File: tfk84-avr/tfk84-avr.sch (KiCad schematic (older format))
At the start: 31 parts, among them J1 USB_C_Receptacle_USB2.0, J2 AVR-ISP-6, SW1 Reset, U1 ATmega32U4-AU, Y1 16MHz

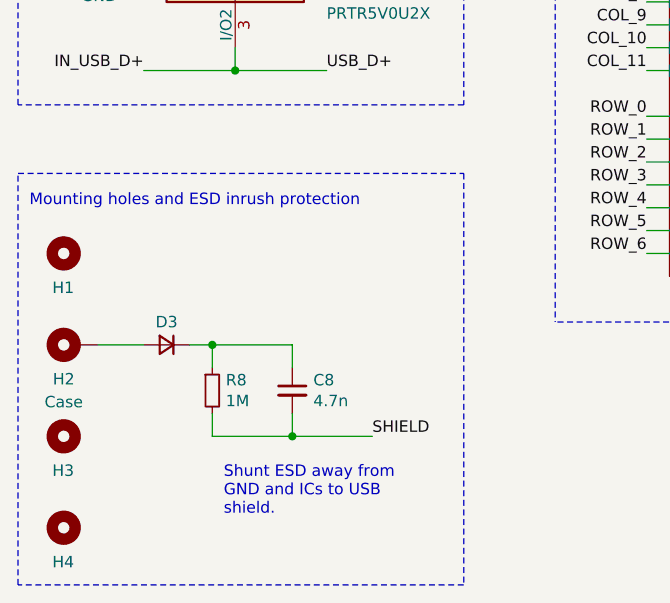
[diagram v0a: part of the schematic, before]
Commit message: Continue layout
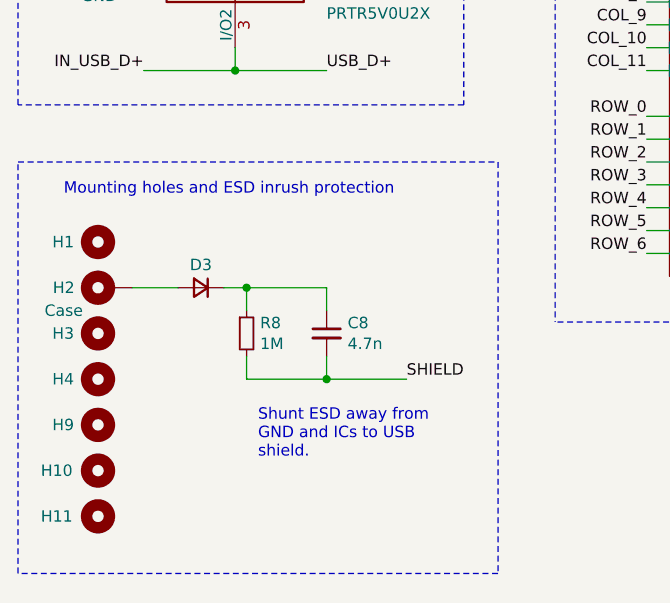
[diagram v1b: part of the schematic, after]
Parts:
- added H10, H11, H9: MountingHole, MountingHole:MountingHole_2.5mm_Pad, symbol Mechanical:MountingHole
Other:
- moved on the sheet: C8, D3, H1, H2, H3, H4, R8
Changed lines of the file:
@@
 L Device:D_Small D3
 U 1 1 60989164
-P 1350 6550
+P 1500 6300
 AR Path="/60989164" Ref="D3"  Part="1"
 AR Path="/60815FFC/60989164" Ref="D?"  Part="1"
-F 0 "D3" H 1350 6450 50  0000 C CNN
-F 1 "Case ESD" H 1350 6434 50  0001 C CNN
-F 2 "Diode_SMD:D_SOD-123" V 1350 6550 50  0001 C CNN
-F 3 "~" V 1350 6550 50  0001 C CNN
-	1    1350 6550
+F 0 "D3" H 1500 6200 50  0000 C CNN
+F 1 "Case ESD" H 1500 6184 50  0001 C CNN
+F 2 "Diode_SMD:D_SOD-123" V 1500 6300 50  0001 C CNN
+F 3 "~" V 1500 6300 50  0001 C CNN
+	1    1500 6300
 	-1   0    0    1
 $EndComp
 Wire Wire Line
-	1450 6550 1550 6550
-Wire Wire Line
-	1550 6550 1550 6650
-Wire Wire Line
-	1550 6550 1900 6550
-Wire Wire Line
-	1900 6550 1900 6650
-Connection ~ 1550 6550
+	1600 6300 1700 6300
+Wire Wire Line
+	1700 6300 1700 6400
+Wire Wire Line
+	1700 6300 2050 6300
+Wire Wire Line
+	2050 6300 2050 6400
+Connection ~ 1700 6300
 $Comp
 L Device:R_Small R8
 U 1 1 6098916F
-P 1550 6750
+P 1700 6500
 AR Path="/6098916F" Ref="R8"  Part="1"
 AR Path="/60815FFC/6098916F" Ref="R?"  Part="1"
-F 0 "R8" H 1609 6796 50  0000 L CNN
-F 1 "1M" H 1609 6705 50  0000 L CNN
-F 2 "Resistor_SMD:R_0805_2012Metric_Pad1.20x1.40mm_HandSolder" H 1550 6750 50  0001 C CNN
-F 3 "~" H 1550 6750 50  0001 C CNN
-	1    1550 6750
+F 0 "R8" H 1759 6546 50  0000 L CNN
+F 1 "1M" H 1759 6455 50  0000 L CNN
+F 2 "Resistor_SMD:R_0805_2012Metric_Pad1.20x1.40mm_HandSolder" H 1700 6500 50  0001 C CNN
+F 3 "~" H 1700 6500 50  0001 C CNN
+	1    1700 6500
 	1    0    0    -1
 $EndComp
@@
 L Device:C_Small C8
 U 1 1 60989175
-P 1900 6750
+P 2050 6500
 AR Path="/60989175" Ref="C8"  Part="1"
 AR Path="/60815FFC/60989175" Ref="C?"  Part="1"
-F 0 "C8" H 1992 6796 50  0000 L CNN
-F 1 "4.7n" H 1992 6705 50  0000 L CNN
-F 2 "Capacitor_SMD:C_0805_2012Metric_Pad1.18x1.45mm_HandSolder" H 1900 6750 50  0001 C CNN
-F 3 "~" H 1900 6750 50  0001 C CNN
-	1    1900 6750
-	1    0    0    -1
-$EndComp
-Wire Wire Line
-	1900 6850 1900 6950
-Wire Wire Line
-	1900 6950 1550 6950
-Wire Wire Line
-	1550 6950 1550 6850
-Text Notes 750  5950 0    50   ~ 0
+F 0 "C8" H 2142 6546 50  0000 L CNN
+F 1 "4.7n" H 2142 6455 50  0000 L CNN
+F 2 "Capacitor_SMD:C_0805_2012Metric_Pad1.18x1.45mm_HandSolder" H 2050 6500 50  0001 C CNN
+F 3 "~" H 2050 6500 50  0001 C CNN
+	1    2050 6500
+	1    0    0    -1
+$EndComp
+Wire Wire Line
+	2050 6600 2050 6700
+Wire Wire Line
+	2050 6700 1700 6700
+Wire Wire Line
+	1700 6700 1700 6600
+Text Notes 900  5900 0    50   ~ 0
 Mounting holes and ESD inrush protection
 Wire Notes Line
-	700  5800 2650 5800
-Wire Notes Line
-	2650 5800 2650 7600
-Wire Notes Line
-	2650 7600 700  7600
-Wire Notes Line
-	700  7600 700  5800
-Wire Wire Line
-	1250 6550 1050 6550
+	700  5750 2800 5750
+Wire Notes Line
+	2800 5750 2800 7550
+Wire Notes Line
+	2800 7550 700  7550
+Wire Notes Line
+	700  7550 700  5750
+Wire Wire Line
+	1400 6300 1200 6300
 $Comp
 L Mechanical:MountingHole_Pad H2
 U 1 1 60989184
-P 950 6550
+P 1100 6300
 AR Path="/60989184" Ref="H2"  Part="1"
 AR Path="/60815FFC/60989184" Ref="H?"  Part="1"
-F 0 "H2" V 800 6600 50  0000 C CNN
-F 1 "Case" V 700 6600 50  0000 C CNN
-F 2 "MountingHole:MountingHole_2.5mm_Pad" H 950 6550 50  0001 C CNN
-F 3 "~" H 950 6550 50  0001 C CNN
-	1    950  6550
+F 0 "H2" V 1100 6500 50  0000 C CNN
+F 1 "Case" V 1000 6500 50  0000 C CNN
+F 2 "MountingHole:MountingHole_2.5mm_Pad" H 1100 6300 50  0001 C CNN
+F 3 "~" H 1100 6300 50  0001 C CNN
+	1    1100 6300
 	0    -1   -1   0
 $EndComp
 Wire Wire Line
-	1900 6950 2250 6950
-Connection ~ 1900 6950
-Text Label 2250 6950 0    50   ~ 0
+	2050 6700 2400 6700
+Connection ~ 2050 6700
+Text Label 2400 6700 0    50   ~ 0
 SHIELD
-Text Notes 1600 7300 0    50   ~ 0
+Text Notes 1750 7050 0    50   ~ 0
 Shunt ESD away from \nGND and ICs to USB \nshield.
 Wire Wire Line
@@
 L Mechanical:MountingHole H1
 U 1 1 60BC9C45
-P 900 6150
-F 0 "H1" H 850 6000 50  0000 L CNN
-F 1 "MountingHole" H 800 5900 50  0001 L CNN
-F 2 "MountingHole:MountingHole_2.5mm_Pad" H 900 6150 50  0001 C CNN
-F 3 "~" H 900 6150 50  0001 C CNN
-	1    900  6150
+P 1050 6100
+F 0 "H1" H 850 6100 50  0000 L CNN
+F 1 "MountingHole" H 950 5850 50  0001 L CNN
+F 2 "MountingHole:MountingHole_2.5mm_Pad" H 1050 6100 50  0001 C CNN
+F 3 "~" H 1050 6100 50  0001 C CNN
+	1    1050 6100
 	1    0    0    -1
 $EndComp
@@
 L Mechanical:MountingHole H3
 U 1 1 60BCA1EE
-P 900 6950
-F 0 "H3" H 850 6800 50  0000 L CNN
-F 1 "MountingHole" H 1000 6905 50  0001 L CNN
-F 2 "MountingHole:MountingHole_2.5mm_Pad" H 900 6950 50  0001 C CNN
-F 3 "~" H 900 6950 50  0001 C CNN
-	1    900  6950
+P 1050 6500
+F 0 "H3" H 850 6500 50  0000 L CNN
+F 1 "MountingHole" H 1150 6455 50  0001 L CNN
+F 2 "MountingHole:MountingHole_2.5mm_Pad" H 1050 6500 50  0001 C CNN
+F 3 "~" H 1050 6500 50  0001 C CNN
+	1    1050 6500
 	1    0    0    -1
 $EndComp
@@
 L Mechanical:MountingHole H4
 U 1 1 60BCA526
-P 900 7350
-F 0 "H4" H 850 7200 50  0000 L CNN
-F 1 "MountingHole" H 1000 7305 50  0001 L CNN
-F 2 "MountingHole:MountingHole_2.5mm_Pad" H 900 7350 50  0001 C CNN
-F 3 "~" H 900 7350 50  0001 C CNN
-	1    900  7350
+P 1050 6700
+F 0 "H4" H 850 6700 50  0000 L CNN
+F 1 "MountingHole" H 1150 6655 50  0001 L CNN
+F 2 "MountingHole:MountingHole_2.5mm_Pad" H 1050 6700 50  0001 C CNN
+F 3 "~" H 1050 6700 50  0001 C CNN
+	1    1050 6700
 	1    0    0    -1
 $EndComp
@@
 Text Label 10150 4650 0    50   ~ 0
 COL_11
+$Comp
+L Mechanical:MountingHole H9
+U 1 1 60FF3666
+P 1050 6900
+F 0 "H9" H 850 6900 50  0000 L CNN
+F 1 "MountingHole" H 1150 6855 50  0001 L CNN
+F 2 "MountingHole:MountingHole_2.5mm_Pad" H 1050 6900 50  0001 C CNN
+F 3 "~" H 1050 6900 50  0001 C CNN
+	1    1050 6900
+	1    0    0    -1
+$EndComp
+$Comp
+L Mechanical:MountingHole H10
+U 1 1 60FF38B8
+P 1050 7100
+F 0 "H10" H 800 7100 50  0000 L CNN
+F 1 "MountingHole" H 1150 7055 50  0001 L CNN
+F 2 "MountingHole:MountingHole_2.5mm_Pad" H 1050 7100 50  0001 C CNN
+F 3 "~" H 1050 7100 50  0001 C CNN
+	1    1050 7100
+	1    0    0    -1
+$EndComp
+$Comp
+L Mechanical:MountingHole H11
+U 1 1 60FF3AA3
+P 1050 7300
+F 0 "H11" H 800 7300 50  0000 L CNN
+F 1 "MountingHole" H 1150 7255 50  0001 L CNN
+F 2 "MountingHole:MountingHole_2.5mm_Pad" H 1050 7300 50  0001 C CNN
+F 3 "~" H 1050 7300 50  0001 C CNN
+	1    1050 7300
+	1    0    0    -1
+$EndComp
 $EndSCHEMATC

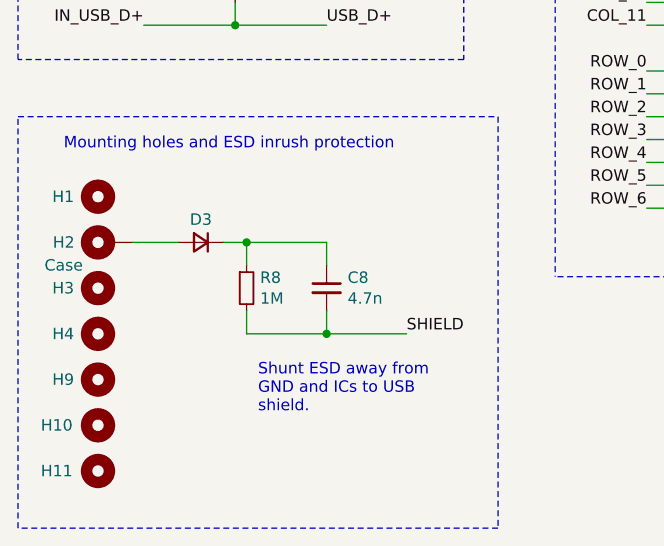
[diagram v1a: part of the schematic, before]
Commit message: Continue layout
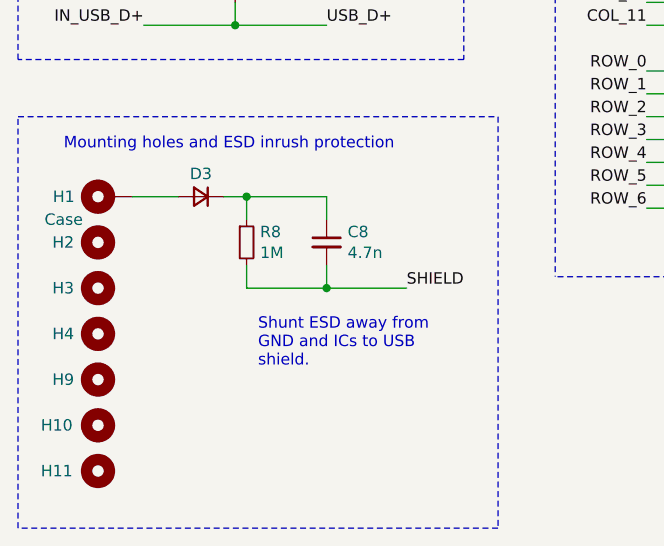
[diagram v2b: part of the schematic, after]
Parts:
- H1: renamed from H2; footprint MountingHole:MountingHole_2.5mm_Pad -> MountingHole:MountingHole_2.5mm_Pad_TopOnly
- H10, H11, H3, H4, H9: footprint MountingHole:MountingHole_2.5mm_Pad -> MountingHole:MountingHole_2.5mm_Pad_TopOnly
- H2: renamed from H1; footprint MountingHole:MountingHole_2.5mm_Pad -> MountingHole:MountingHole_2.5mm_Pad_TopOnly
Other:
- moved on the sheet: C8, D3, H1, H2, R8
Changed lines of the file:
@@
 L Device:D_Small D3
 U 1 1 60989164
-P 1500 6300
+P 1500 6100
 AR Path="/60989164" Ref="D3"  Part="1"
 AR Path="/60815FFC/60989164" Ref="D?"  Part="1"
-F 0 "D3" H 1500 6200 50  0000 C CNN
-F 1 "Case ESD" H 1500 6184 50  0001 C CNN
-F 2 "Diode_SMD:D_SOD-123" V 1500 6300 50  0001 C CNN
-F 3 "~" V 1500 6300 50  0001 C CNN
-	1    1500 6300
+F 0 "D3" H 1500 6000 50  0000 C CNN
+F 1 "Case ESD" H 1500 5984 50  0001 C CNN
+F 2 "Diode_SMD:D_SOD-123" V 1500 6100 50  0001 C CNN
+F 3 "~" V 1500 6100 50  0001 C CNN
+	1    1500 6100
 	-1   0    0    1
 $EndComp
 Wire Wire Line
-	1600 6300 1700 6300
-Wire Wire Line
-	1700 6300 1700 6400
-Wire Wire Line
-	1700 6300 2050 6300
-Wire Wire Line
-	2050 6300 2050 6400
-Connection ~ 1700 6300
+	1600 6100 1700 6100
+Wire Wire Line
+	1700 6100 1700 6200
+Wire Wire Line
+	1700 6100 2050 6100
+Wire Wire Line
+	2050 6100 2050 6200
+Connection ~ 1700 6100
 $Comp
 L Device:R_Small R8
 U 1 1 6098916F
-P 1700 6500
+P 1700 6300
 AR Path="/6098916F" Ref="R8"  Part="1"
 AR Path="/60815FFC/6098916F" Ref="R?"  Part="1"
-F 0 "R8" H 1759 6546 50  0000 L CNN
-F 1 "1M" H 1759 6455 50  0000 L CNN
-F 2 "Resistor_SMD:R_0805_2012Metric_Pad1.20x1.40mm_HandSolder" H 1700 6500 50  0001 C CNN
-F 3 "~" H 1700 6500 50  0001 C CNN
-	1    1700 6500
+F 0 "R8" H 1759 6346 50  0000 L CNN
+F 1 "1M" H 1759 6255 50  0000 L CNN
+F 2 "Resistor_SMD:R_0805_2012Metric_Pad1.20x1.40mm_HandSolder" H 1700 6300 50  0001 C CNN
+F 3 "~" H 1700 6300 50  0001 C CNN
+	1    1700 6300
 	1    0    0    -1
 $EndComp
@@
 L Device:C_Small C8
 U 1 1 60989175
-P 2050 6500
+P 2050 6300
 AR Path="/60989175" Ref="C8"  Part="1"
 AR Path="/60815FFC/60989175" Ref="C?"  Part="1"
-F 0 "C8" H 2142 6546 50  0000 L CNN
-F 1 "4.7n" H 2142 6455 50  0000 L CNN
-F 2 "Capacitor_SMD:C_0805_2012Metric_Pad1.18x1.45mm_HandSolder" H 2050 6500 50  0001 C CNN
-F 3 "~" H 2050 6500 50  0001 C CNN
-	1    2050 6500
-	1    0    0    -1
-$EndComp
-Wire Wire Line
-	2050 6600 2050 6700
-Wire Wire Line
-	2050 6700 1700 6700
-Wire Wire Line
-	1700 6700 1700 6600
+F 0 "C8" H 2142 6346 50  0000 L CNN
+F 1 "4.7n" H 2142 6255 50  0000 L CNN
+F 2 "Capacitor_SMD:C_0805_2012Metric_Pad1.18x1.45mm_HandSolder" H 2050 6300 50  0001 C CNN
+F 3 "~" H 2050 6300 50  0001 C CNN
+	1    2050 6300
+	1    0    0    -1
+$EndComp
+Wire Wire Line
+	2050 6400 2050 6500
+Wire Wire Line
+	2050 6500 1700 6500
+Wire Wire Line
+	1700 6500 1700 6400
 Text Notes 900  5900 0    50   ~ 0
 Mounting holes and ESD inrush protection
@@
 	700  7550 700  5750
 Wire Wire Line
-	1400 6300 1200 6300
-$Comp
-L Mechanical:MountingHole_Pad H2
+	1400 6100 1200 6100
+$Comp
+L Mechanical:MountingHole_Pad H1
 U 1 1 60989184
-P 1100 6300
-AR Path="/60989184" Ref="H2"  Part="1"
+P 1100 6100
+AR Path="/60989184" Ref="H1"  Part="1"
 AR Path="/60815FFC/60989184" Ref="H?"  Part="1"
-F 0 "H2" V 1100 6500 50  0000 C CNN
-F 1 "Case" V 1000 6500 50  0000 C CNN
-F 2 "MountingHole:MountingHole_2.5mm_Pad" H 1100 6300 50  0001 C CNN
-F 3 "~" H 1100 6300 50  0001 C CNN
-	1    1100 6300
+F 0 "H1" V 1100 6300 50  0000 C CNN
+F 1 "Case" V 1000 6300 50  0000 C CNN
+F 2 "MountingHole:MountingHole_2.5mm_Pad_TopOnly" H 1100 6100 50  0001 C CNN
+F 3 "~" H 1100 6100 50  0001 C CNN
+	1    1100 6100
 	0    -1   -1   0
 $EndComp
 Wire Wire Line
-	2050 6700 2400 6700
-Connection ~ 2050 6700
-Text Label 2400 6700 0    50   ~ 0
+	2050 6500 2400 6500
+Connection ~ 2050 6500
+Text Label 2400 6500 0    50   ~ 0
 SHIELD
-Text Notes 1750 7050 0    50   ~ 0
+Text Notes 1750 6850 0    50   ~ 0
 Shunt ESD away from \nGND and ICs to USB \nshield.
 Wire Wire Line
@@
 	3000 1250 2400 1250
 $Comp
-L Mechanical:MountingHole H1
+L Mechanical:MountingHole H2
 U 1 1 60BC9C45
-P 1050 6100
-F 0 "H1" H 850 6100 50  0000 L CNN
-F 1 "MountingHole" H 950 5850 50  0001 L CNN
-F 2 "MountingHole:MountingHole_2.5mm_Pad" H 1050 6100 50  0001 C CNN
-F 3 "~" H 1050 6100 50  0001 C CNN
-	1    1050 6100
+P 1050 6300
+F 0 "H2" H 850 6300 50  0000 L CNN
+F 1 "MountingHole" H 950 6050 50  0001 L CNN
+F 2 "MountingHole:MountingHole_2.5mm_Pad_TopOnly" H 1050 6300 50  0001 C CNN
+F 3 "~" H 1050 6300 50  0001 C CNN
+	1    1050 6300
 	1    0    0    -1
 $EndComp
@@
 F 0 "H3" H 850 6500 50  0000 L CNN
 F 1 "MountingHole" H 1150 6455 50  0001 L CNN
-F 2 "MountingHole:MountingHole_2.5mm_Pad" H 1050 6500 50  0001 C CNN
+F 2 "MountingHole:MountingHole_2.5mm_Pad_TopOnly" H 1050 6500 50  0001 C CNN
 F 3 "~" H 1050 6500 50  0001 C CNN
 	1    1050 6500
@@
 F 0 "H4" H 850 6700 50  0000 L CNN
 F 1 "MountingHole" H 1150 6655 50  0001 L CNN
-F 2 "MountingHole:MountingHole_2.5mm_Pad" H 1050 6700 50  0001 C CNN
+F 2 "MountingHole:MountingHole_2.5mm_Pad_TopOnly" H 1050 6700 50  0001 C CNN
 F 3 "~" H 1050 6700 50  0001 C CNN
 	1    1050 6700
@@
 F 0 "H9" H 850 6900 50  0000 L CNN
 F 1 "MountingHole" H 1150 6855 50  0001 L CNN
-F 2 "MountingHole:MountingHole_2.5mm_Pad" H 1050 6900 50  0001 C CNN
+F 2 "MountingHole:MountingHole_2.5mm_Pad_TopOnly" H 1050 6900 50  0001 C CNN
 F 3 "~" H 1050 6900 50  0001 C CNN
 	1    1050 6900
@@
 F 0 "H10" H 800 7100 50  0000 L CNN
 F 1 "MountingHole" H 1150 7055 50  0001 L CNN
-F 2 "MountingHole:MountingHole_2.5mm_Pad" H 1050 7100 50  0001 C CNN
+F 2 "MountingHole:MountingHole_2.5mm_Pad_TopOnly" H 1050 7100 50  0001 C CNN
 F 3 "~" H 1050 7100 50  0001 C CNN
 	1    1050 7100
@@
 F 0 "H11" H 800 7300 50  0000 L CNN
 F 1 "MountingHole" H 1150 7255 50  0001 L CNN
-F 2 "MountingHole:MountingHole_2.5mm_Pad" H 1050 7300 50  0001 C CNN
+F 2 "MountingHole:MountingHole_2.5mm_Pad_TopOnly" H 1050 7300 50  0001 C CNN
 F 3 "~" H 1050 7300 50  0001 C CNN
 	1    1050 7300
